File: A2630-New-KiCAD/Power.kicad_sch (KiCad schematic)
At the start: 22 parts, among them U204 74HCT04, U300 74HCT05, U307 74HCT04, U606 74HCT244, U800 LM1117-3.3

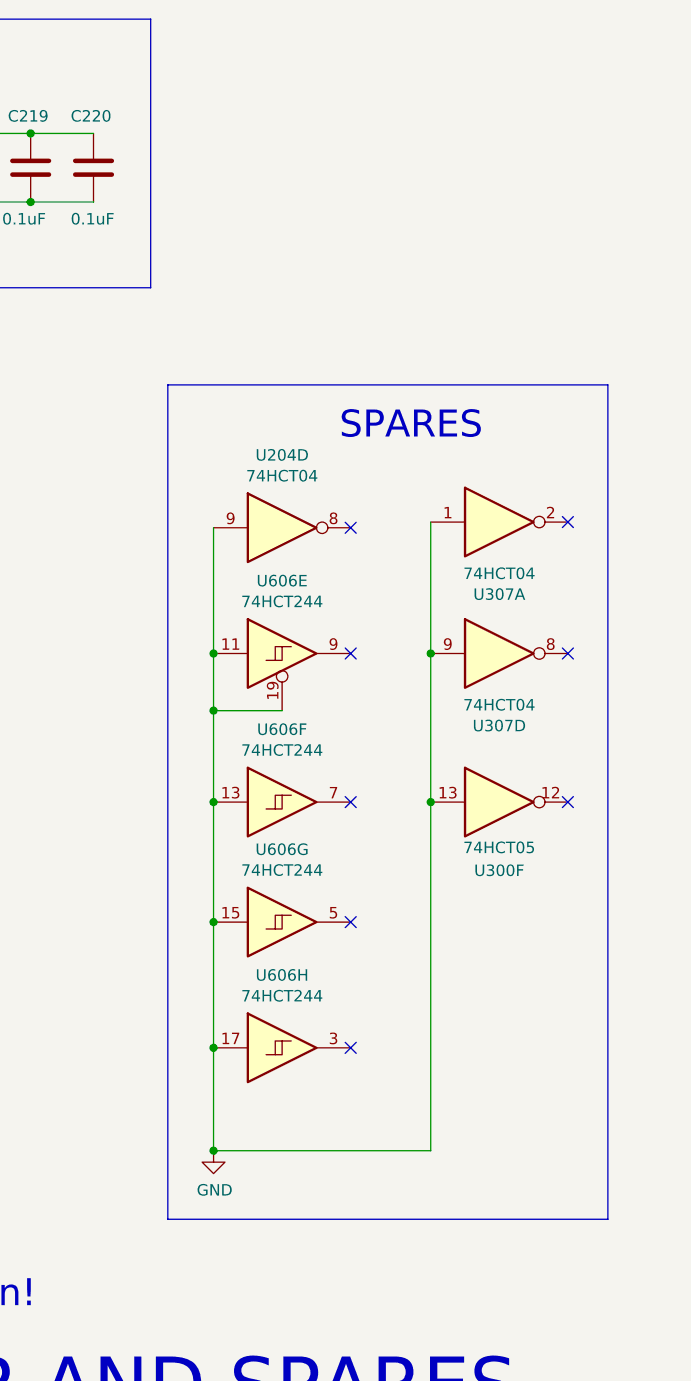
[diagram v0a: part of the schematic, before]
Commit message: Add files via upload
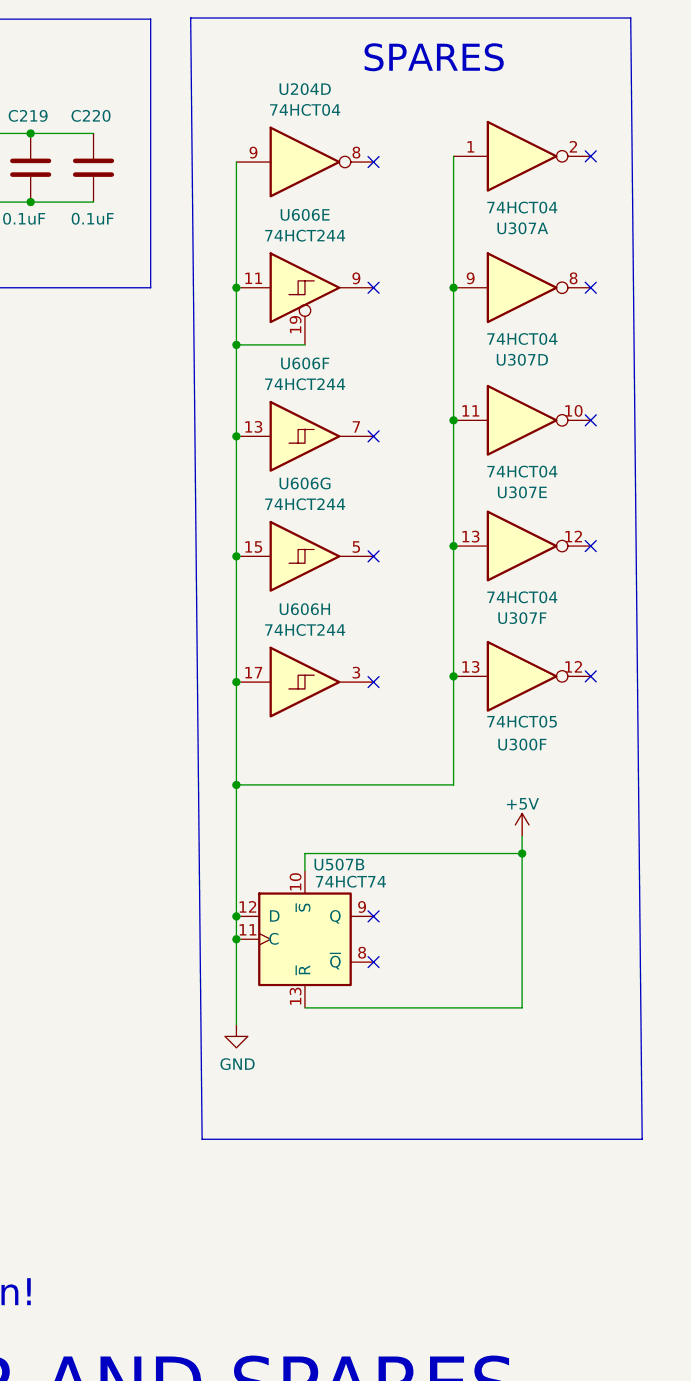
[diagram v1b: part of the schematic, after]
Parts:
- added unit 5 of U307
- added unit 6 of U307
- added U507: 74HCT74, Package_SO:SOIC-14_3.9x8.7mm_P1.27mm, symbol 74xx:74LS74
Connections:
- net +5V: now also U507.10 (~{S}), U507.13 (~{R})
- net GND: now also U307.11, U307.13, U507.11 (C), U507.12 (D)
- no-connect marks 8 -> 12
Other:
- moved on the sheet: U204D, U300F, U307A, U307D, U606E, U606F, U606G, U606H
